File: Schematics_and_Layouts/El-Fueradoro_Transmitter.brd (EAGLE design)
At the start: 91.4 x 66 mm, 58 parts, among them IC1 MAX202, IC2 MEGA168P/328P, IC3 LM3940IT-3.3, Q1 9.8304

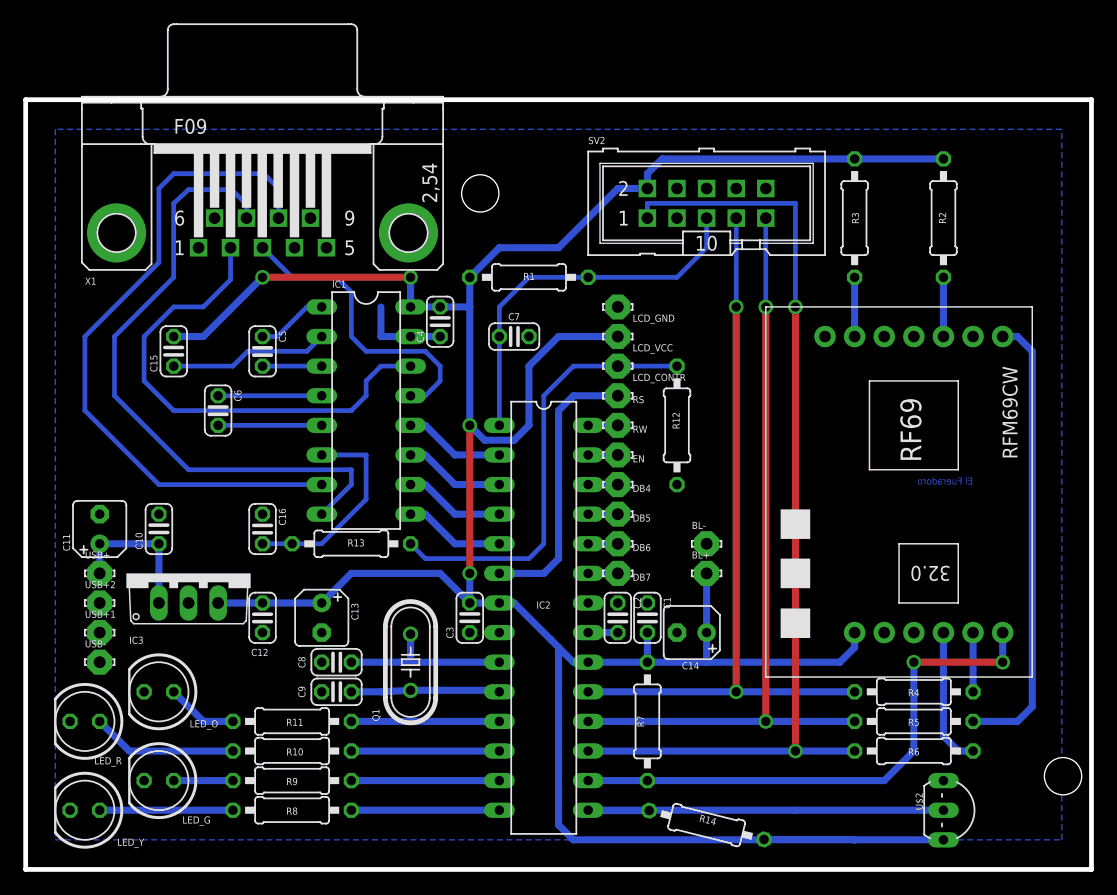
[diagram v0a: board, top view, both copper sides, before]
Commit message: Added Gerber Files
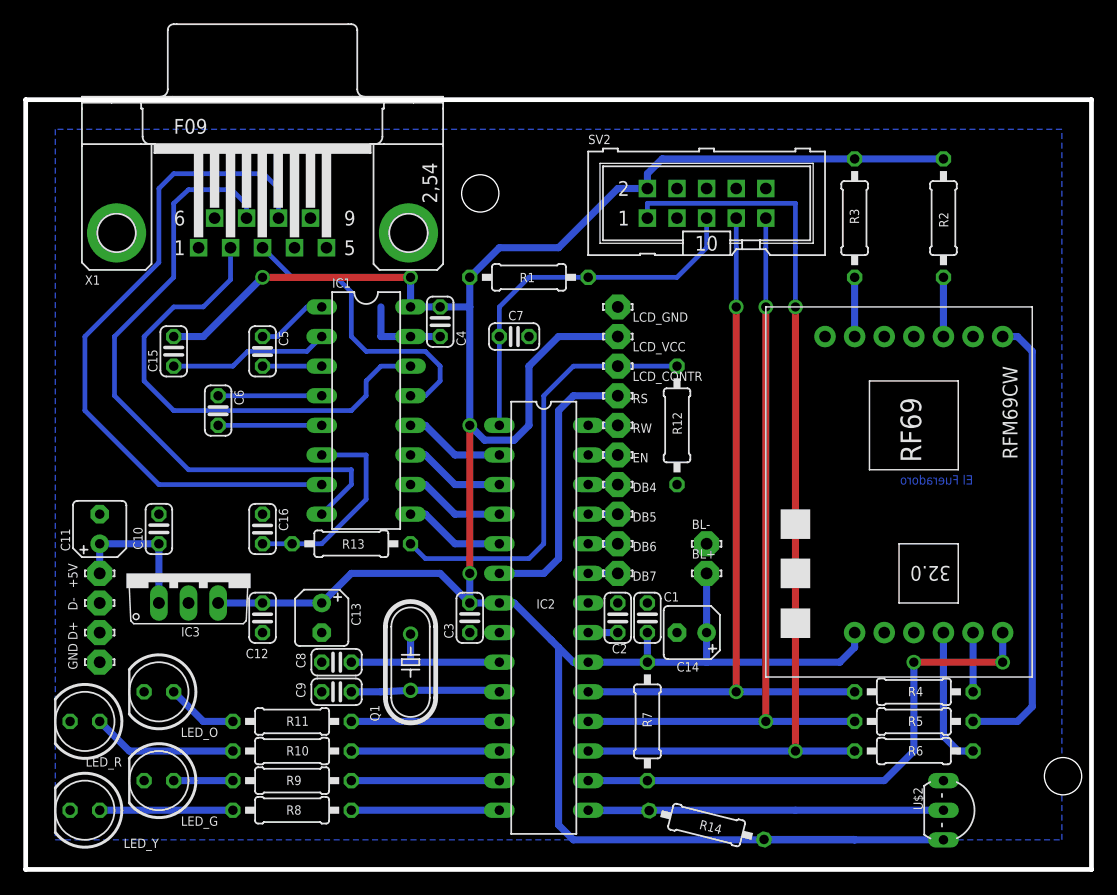
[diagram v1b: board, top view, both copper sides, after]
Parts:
- renumbered USB+ to +5V, USB+1 to D+, USB+2 to D-, USB- to GND
